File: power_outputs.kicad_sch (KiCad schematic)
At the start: 10 parts, among them Q1 BSS138, Q3 MMBT3904, Q4 MMBT3906

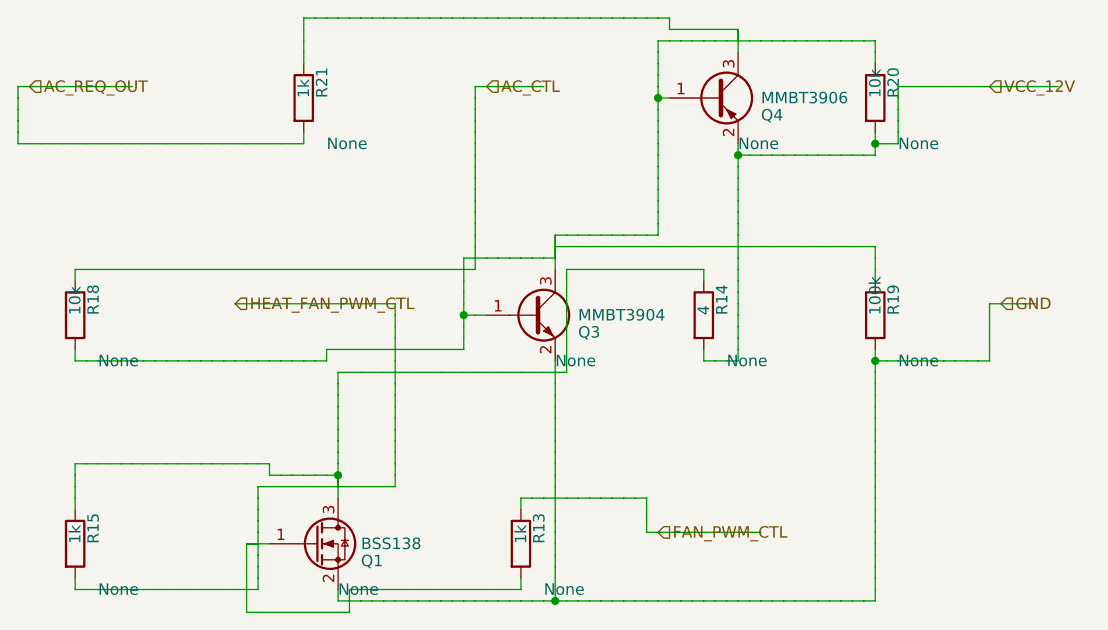
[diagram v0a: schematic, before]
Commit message: рефакторинг проекта и начала прогона тестов
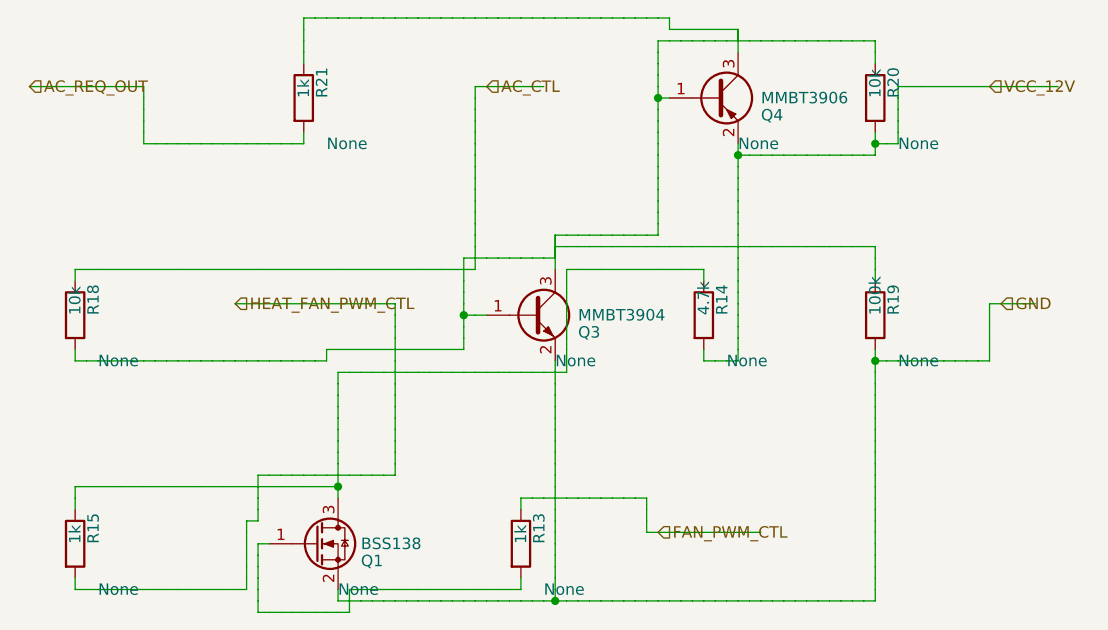
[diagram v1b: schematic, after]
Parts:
- R14: value 4 -> 4.7k
